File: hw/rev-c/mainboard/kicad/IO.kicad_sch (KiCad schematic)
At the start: 7 parts, among them U11 W65C21N, U12 W65C21N, U13 W65C22N

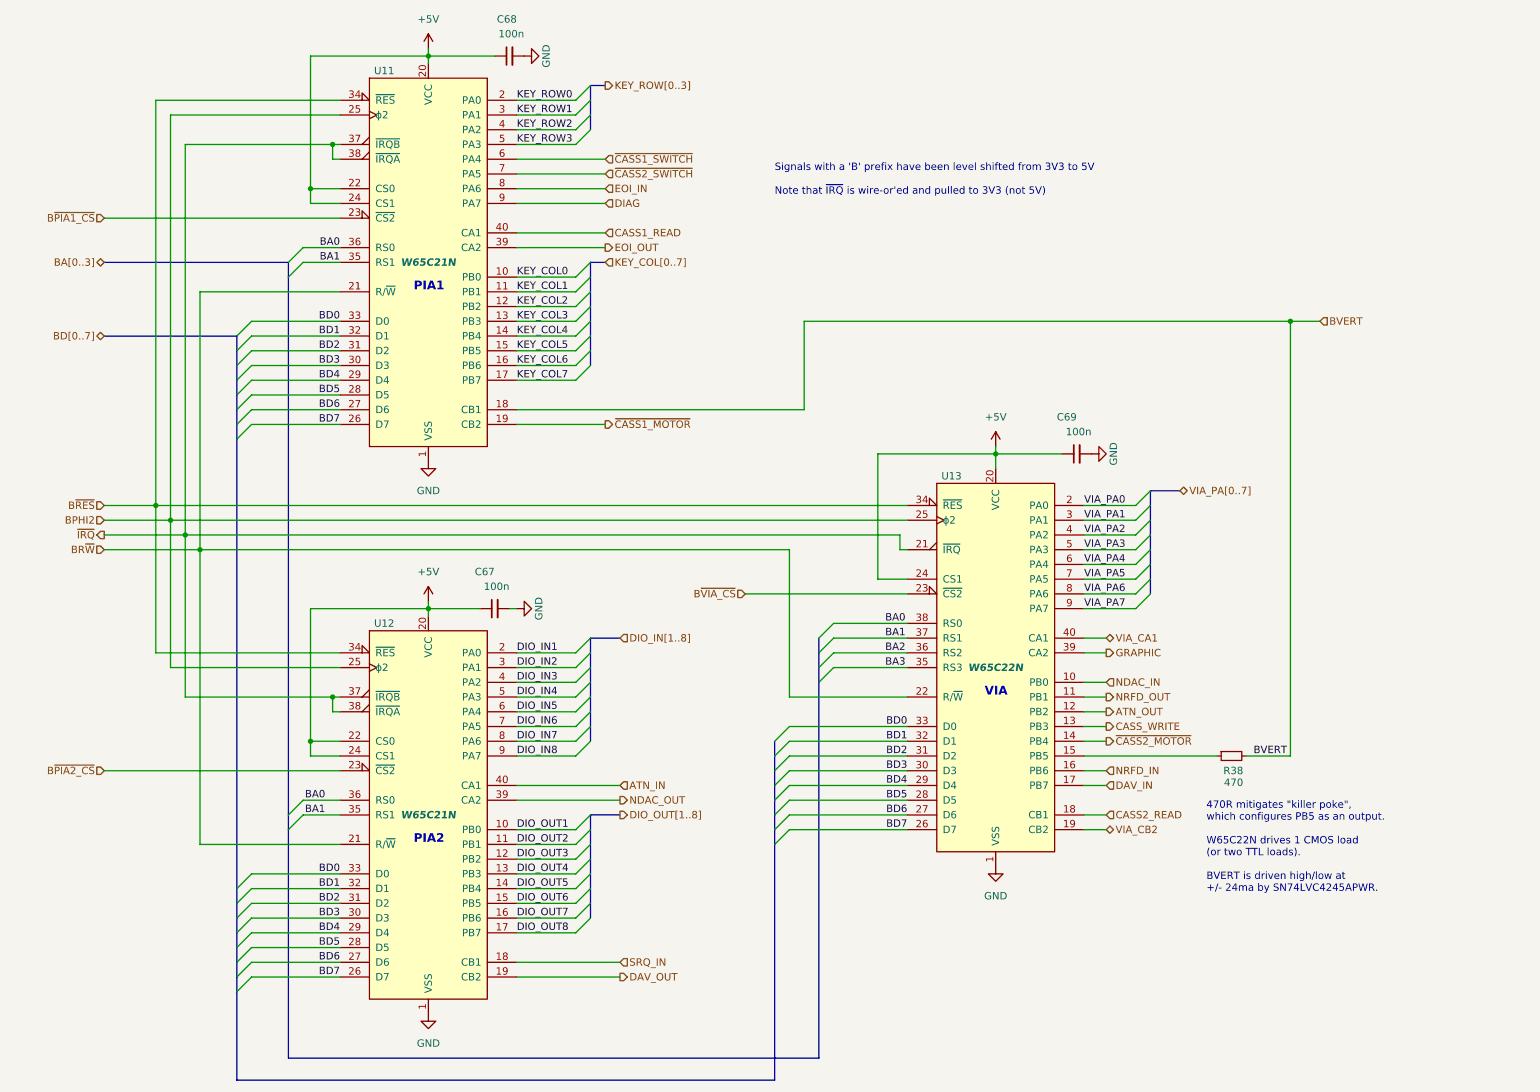
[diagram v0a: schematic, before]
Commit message: hw: tidy
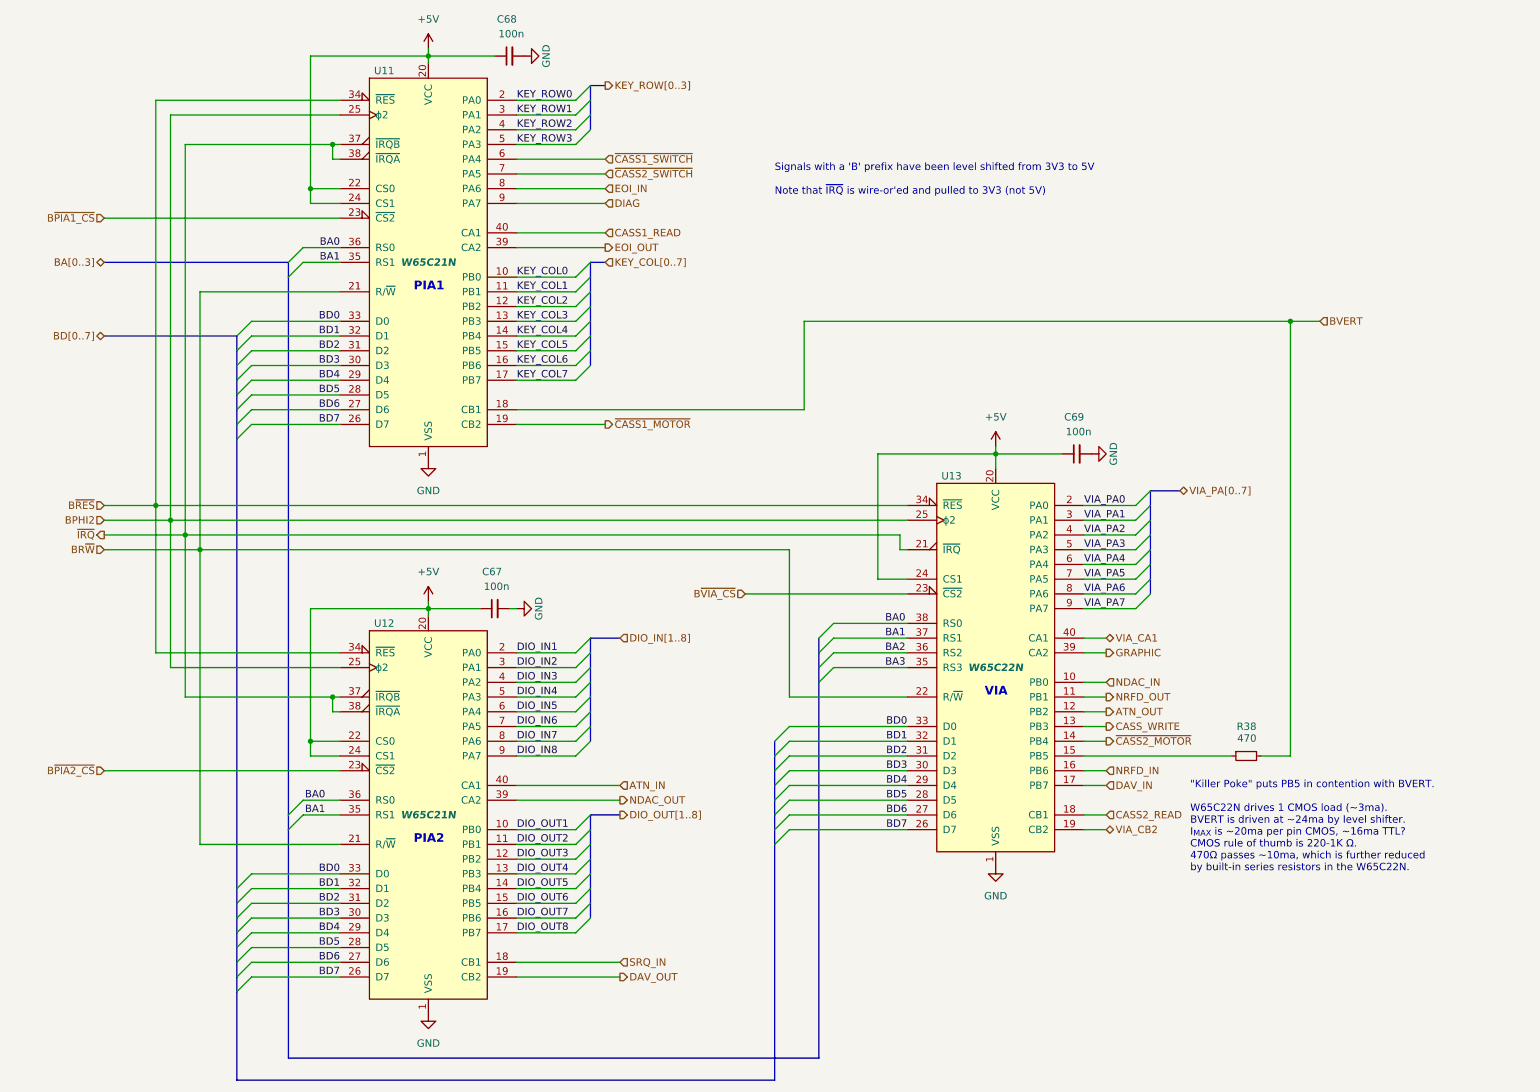
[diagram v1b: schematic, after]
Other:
- note added: ""Killer Poke" puts PB5 in contention with BVERT. W65C22N drives 1 CMOS load (~3ma). BVERT is driven at ~24ma by level shifter. I_{MAX} is ~20ma per pin CMOS, ~16ma TTL? CMOS rule of thumb is 220-1K Ω. 470Ω passes ~10ma, which is further reduced by built-in series resistors in the W65C22N."
- note removed: "470R mitigates "killer poke", which configures PB5 as an output. W65C22N drives 1 CMOS load (or two TTL loads). BVERT is driven high/low at +/- 24ma by SN74LVC4245APWR."
- moved on the sheet: R38
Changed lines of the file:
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@@
 	(wire
 		(pts
-			(xy 199.39 143.51) (xy 222.25 143.51)
+			(xy 199.39 143.51) (xy 224.79 143.51)
 		)
 		(stroke
@@
 	(wire
 		(pts
-			(xy 227.33 143.51) (xy 234.95 143.51)
+			(xy 229.87 143.51) (xy 234.95 143.51)
 		)
 		(stroke
@@
 		)
 	)
-	(text "470R mitigates \"killer poke\",\nwhich configures PB5 as an output.\n\nW65C22N drives 1 CMOS load\n(or two TTL loads).\n\nBVERT is driven high/low at\n+/- 24ma by SN74LVC4245APWR."
+	(text "\"Killer Poke\" puts PB5 in contention with BVERT.\n\nW65C22N drives 1 CMOS load (~3ma).\nBVERT is driven at ~24ma by level shifter.\nI_{MAX} is ~20ma per pin CMOS, ~16ma TTL?\nCMOS rule of thumb is 220-1K Ω.\n470Ω passes ~10ma, which is further reduced\nby built-in series resistors in the W65C22N."
 		(exclude_from_sim no)
-		(at 220.472 159.258 0)
+		(at 217.678 155.702 0)
 		(effects
 			(font
@@
 	(label "DIO_IN4"
 		(at 101.6 133.35 0)
-		(fields_autoplaced yes)
-		(effects
-			(font
-				(size 1.27 1.27)
-			)
-			(justify left bottom)
-		)
-	)
-	(label "BVERT"
-		(at 228.6 143.51 0)
 		(fields_autoplaced yes)
 		(effects
@@
 		(dnp no)
 		(property "Reference" "C67"
-			(at 97.79 111.76 90)
+			(at 99.06 111.76 90)
 			(effects
 				(font
@@
 		(dnp no)
 		(property "Reference" "C69"
-			(at 198.12 85.09 90)
+			(at 199.39 85.09 90)
 			(effects
 				(font
@@
 	(symbol
 		(lib_id "Device:R_Small")
-		(at 224.79 143.51 90)
+		(at 227.33 143.51 90)
 		(mirror x)
 		(unit 1)
@@
 		(dnp no)
 		(property "Reference" "R38"
-			(at 226.822 146.05 90)
+			(at 229.108 138.43 90)
 			(effects
 				(font
@@
 		)
 		(property "Value" "470"
-			(at 226.822 148.082 90)
+			(at 229.108 140.462 90)
 			(effects
 				(font
@@
 		)
 		(property "Footprint" "Resistor_SMD:R_0402_1005Metric"
-			(at 224.79 143.51 0)
+			(at 227.33 143.51 0)
 			(effects
 				(font
@@
 			)
 		)
-		(property "Datasheet" "https://datasheet.lcsc.com/lcsc/2205311900_UNI-ROYAL-Uniroyal-Elec-0402WGF4700TCE_C25117.pdf"
-			(at 224.79 143.51 0)
+		(property "Datasheet" ""
+			(at 227.33 143.51 0)
 			(effects
 				(font
@@
 		)
 		(property "Description" ""
-			(at 224.79 143.51 0)
+			(at 227.33 143.51 0)
 			(effects
 				(font
@@
 		)
 		(property "LCSC" "C25117"
-			(at 224.79 143.51 0)
-			(effects
-				(font
+			(at 227.33 143.51 0)
+			(effects
+				(font
